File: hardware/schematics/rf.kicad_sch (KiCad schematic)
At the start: 46 parts, among them IC8 SI4468-A2A-IMR, J5 RFPC-SMA28-F, Q6 DMN1008UFDF-7

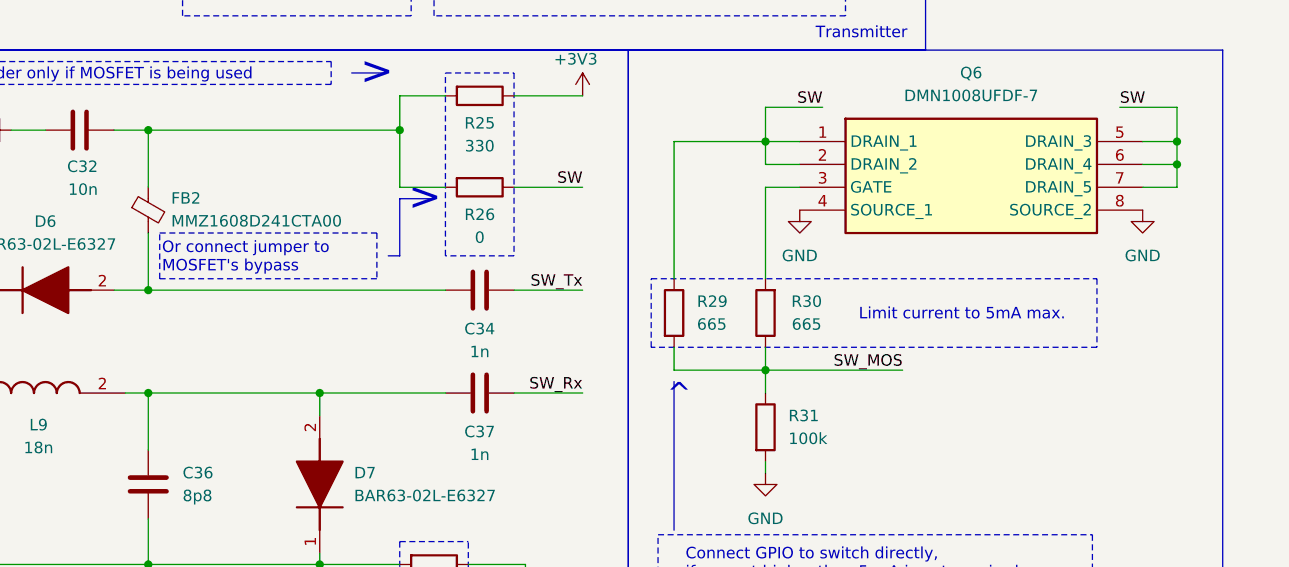
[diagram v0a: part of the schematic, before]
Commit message: gitignore added
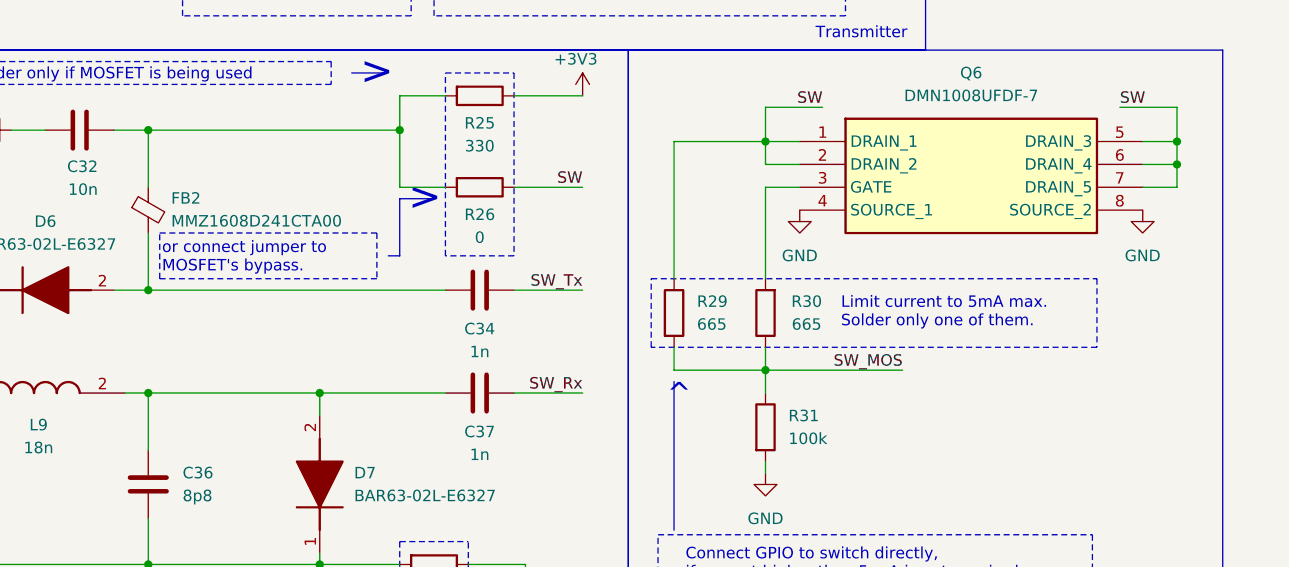
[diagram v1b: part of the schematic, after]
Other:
- note added: "Limit current to 5mA max. Solder only one of them."
- note added: "or connect jumper to MOSFET's bypass."
- note removed: "Limit current to 5mA max."
- note removed: "Or connect jumper to MOSFET's bypass"
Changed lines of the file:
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@@
 		)
 	)
-	(text "Or connect jumper to \nMOSFET's bypass"
+	(text "or connect jumper to \nMOSFET's bypass."
 		(exclude_from_sim no)
 		(at 58.674 152.654 0)
@@
 		)
 	)
-	(text "Limit current to 5mA max."
+	(text "Limit current to 5mA max.\nSolder only one of them."
 		(exclude_from_sim no)
-		(at 147.574 159.004 0)
+		(at 134.112 158.75 0)
 		(effects
 			(font
 				(size 1.27 1.27)
 			)
+			(justify left)
 		)
 	)
